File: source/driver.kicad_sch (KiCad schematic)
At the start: 77 parts, among them J4 on/off, P1 SWD, P10 SWD, P2 SWD, P3 SWD, P4 SWD, P5 SWD, P6 SWD, P7 SWD, P8 SWD, P9 SWD, Q1 AO3401A, Q2 SS8050, Q3 SS8050, SW2 SW_DPDT_x2, U3 AMS1117-3.3, U4 IRS21867S, U5 XL1509-5.0E1, U6 IRS21867S, U7 IRS21867S, U8 TX4130L/PW2902

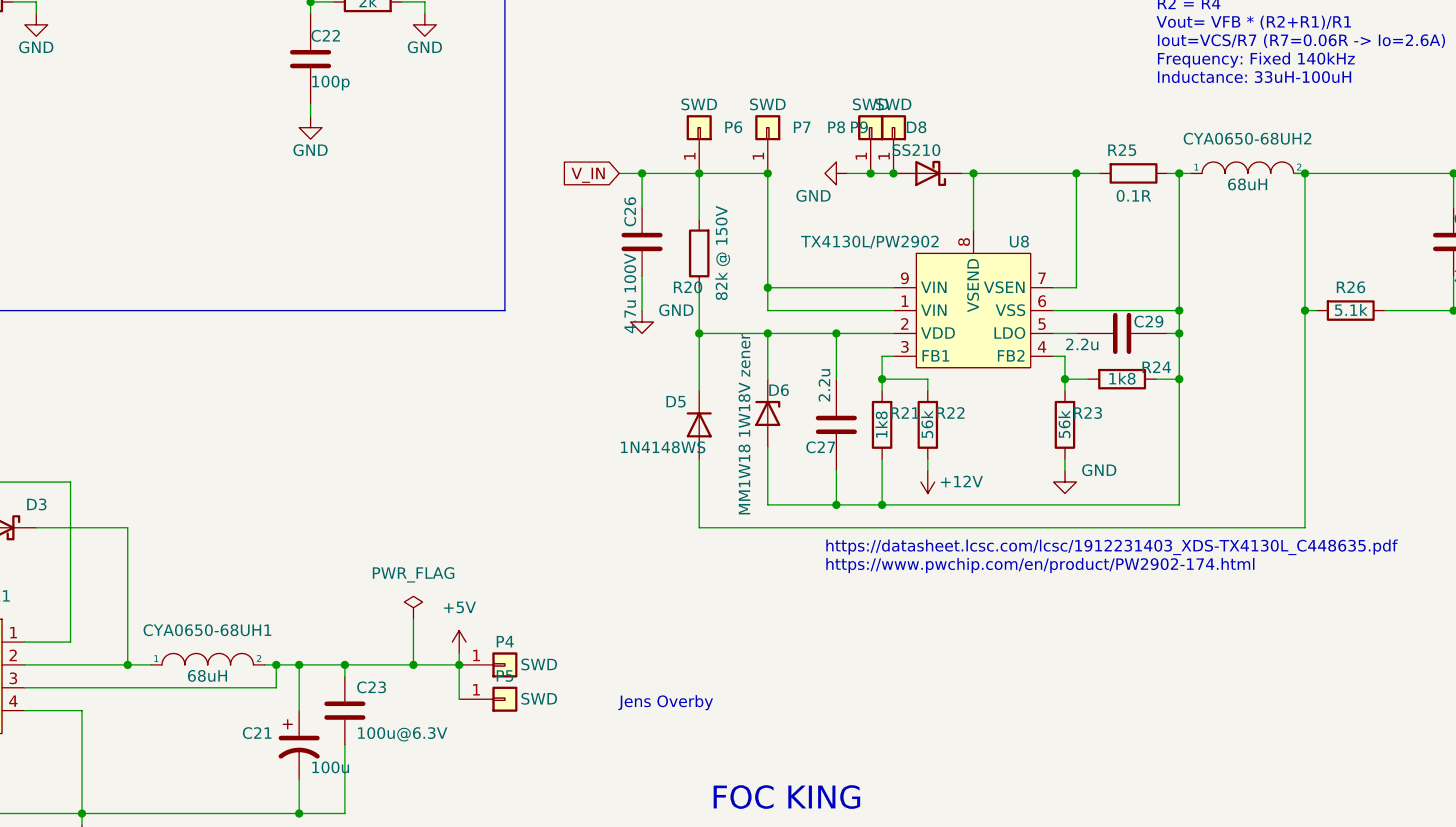
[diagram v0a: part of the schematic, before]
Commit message: update IMU
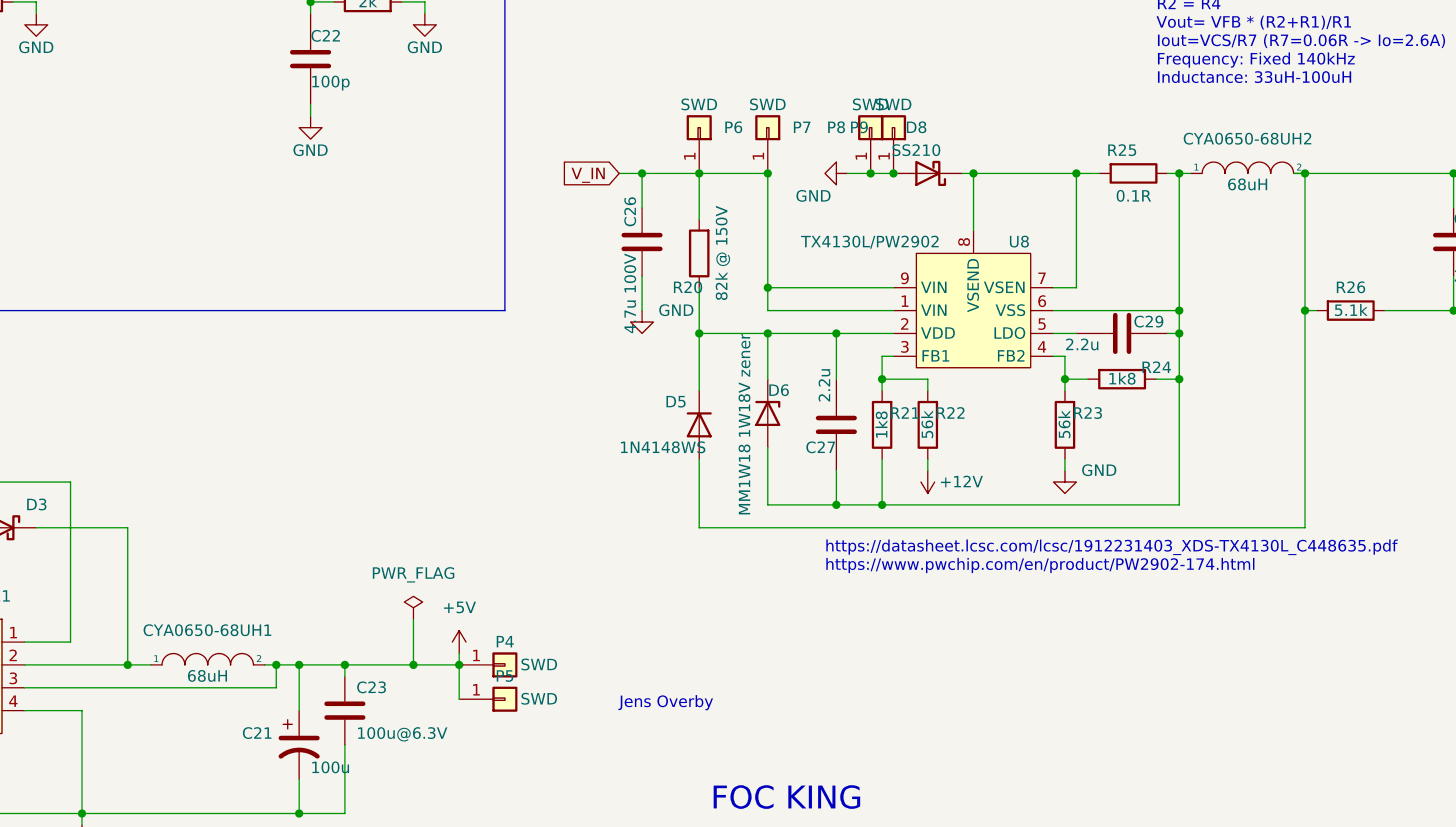
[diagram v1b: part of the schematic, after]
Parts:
- D2, D4, D7: footprint Diode_SMD:D_SMA -> Diode_SMD:D_SOD-123
- D3: footprint Diode_SMD:D_SOD-323 -> Diode_THT:D_DO-41_SOD81_P10.16mm_Horizontal
- D5: footprint Diode_SMD:D_SOD-323 -> Diode_SMD:D_SOD-123
- U8: symbol Custom_Library:TX4130L / PW2902 -> Custom_Library:TX4130L / PW2902
